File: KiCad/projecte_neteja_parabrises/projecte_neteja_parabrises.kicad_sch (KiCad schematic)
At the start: 0 parts

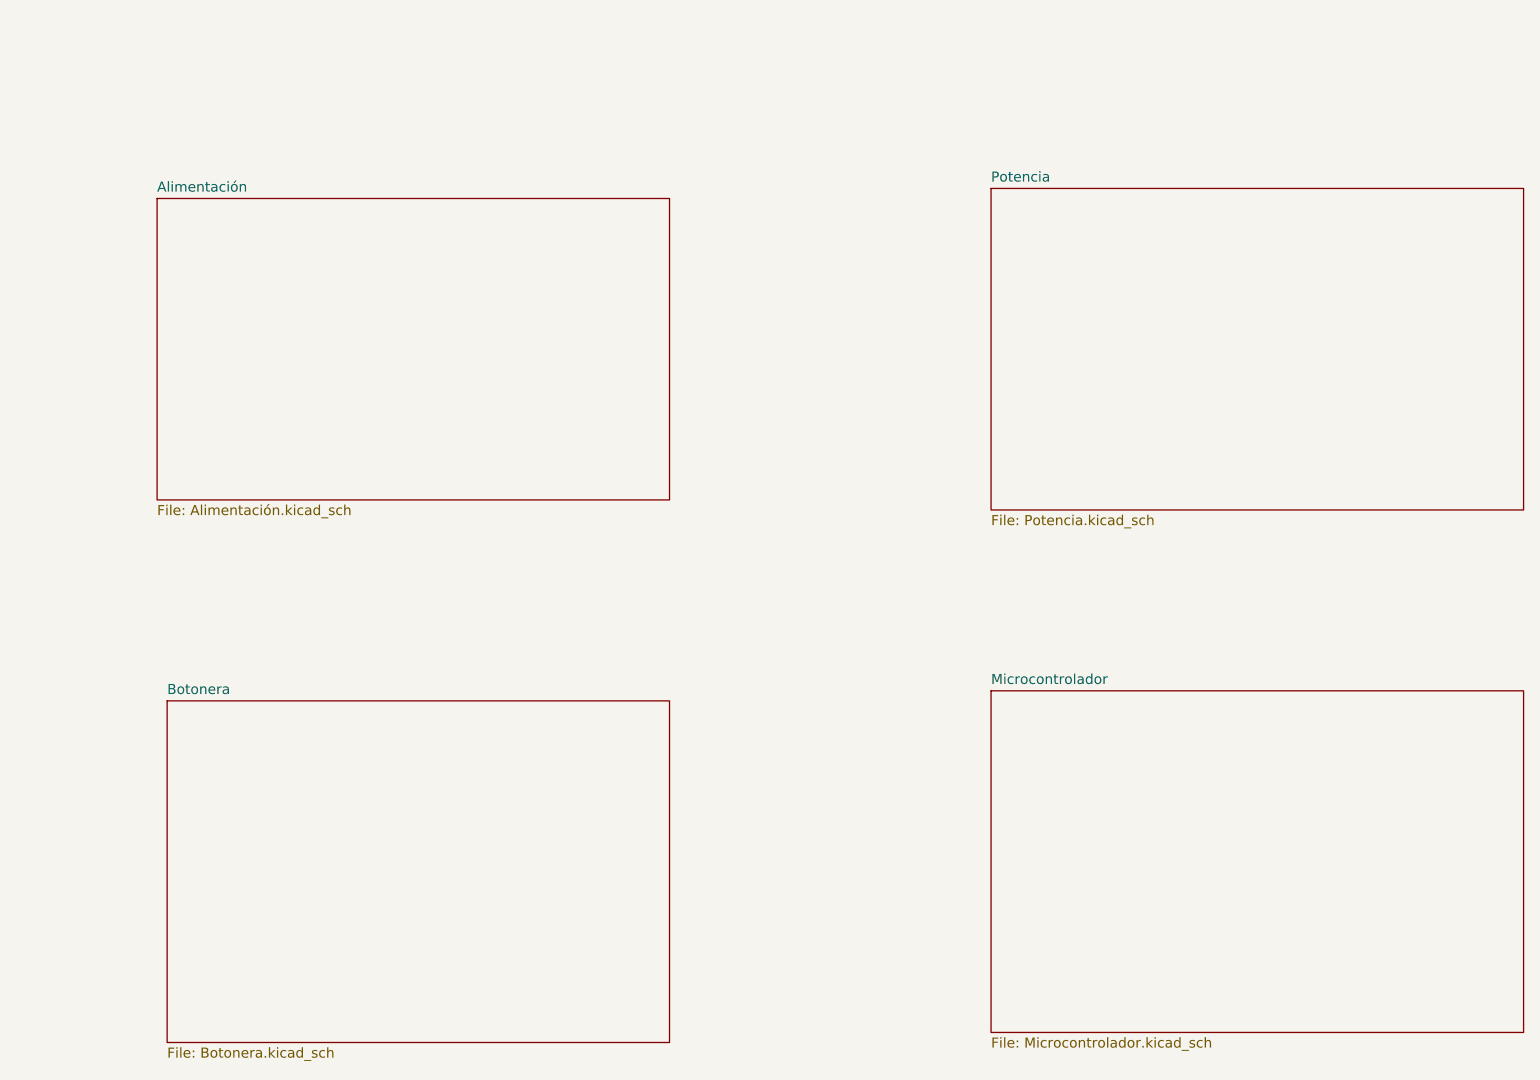
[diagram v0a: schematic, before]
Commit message: ESQUEMATICO V2
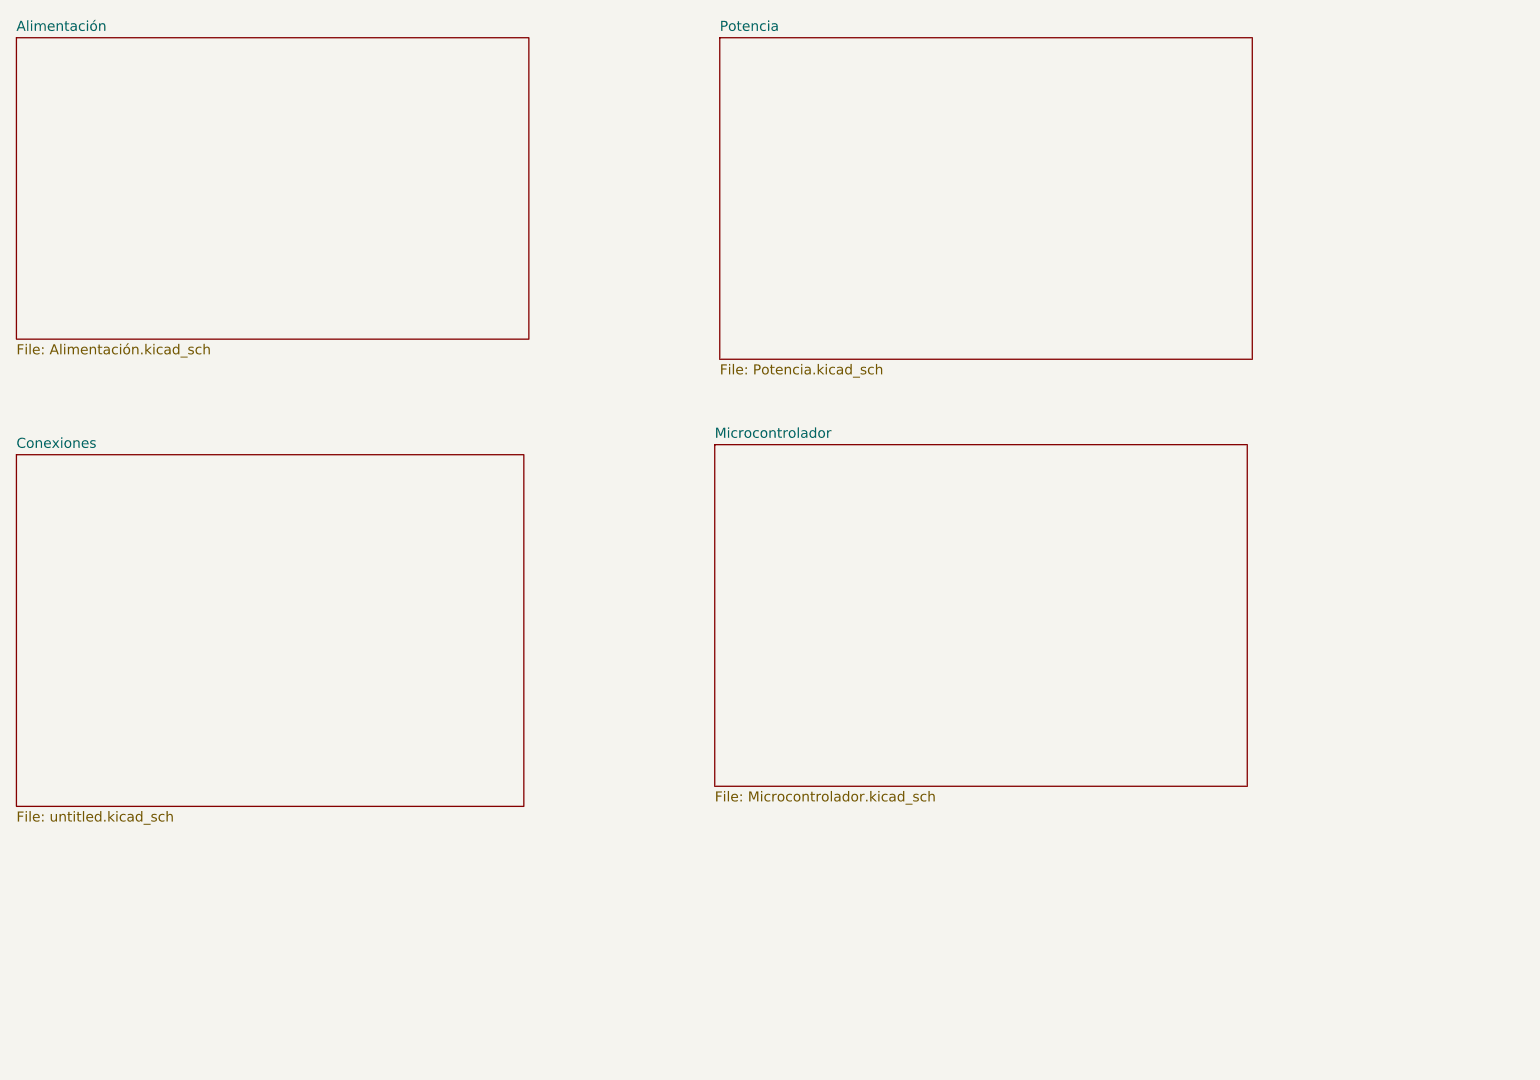
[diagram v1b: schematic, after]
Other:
- removed sheet Botonera
- added sheet Conexiones (untitled.kicad_sch)
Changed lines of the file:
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@@
 	(paper "A4")
 	(sheet
-		(at 40.64 105.41)
-		(size 63.5 43.18)
+		(at 21.59 74.295)
+		(size 64.135 44.45)
 		(exclude_from_sim no)
 		(in_bom yes)
@@
 			(color 0 0 0 0.0000)
 		)
-		(property "Sheetname" "Botonera"
-			(at 40.64 104.6984 0)
+		(property "Sheetname" "Conexiones"
+			(at 21.59 73.5834 0)
 			(effects
 				(font
@@
 			)
 		)
-		(property "Sheetfile" "Botonera.kicad_sch"
-			(at 40.64 149.1746 0)
+		(property "Sheetfile" "untitled.kicad_sch"
+			(at 21.59 119.3296 0)
 			(effects
 				(font
@@
 			)
 		)
+		(property "Field2" ""
+			(at 21.59 74.295 0)
+			(effects
+				(font
+					(size 1.27 1.27)
+				)
+			)
+		)
+		(property "Field3" ""
+			(at 21.59 74.295 0)
+			(effects
+				(font
+					(size 1.27 1.27)
+				)
+			)
+		)
+		(property "Field4" ""
+			(at 21.59 74.295 0)
+			(effects
+				(font
+					(size 1.27 1.27)
+				)
+			)
+		)
+		(property "Field5" ""
+			(at 21.59 74.295 0)
+			(effects
+				(font
+					(size 1.27 1.27)
+				)
+			)
+		)
+		(property "Field6" ""
+			(at 21.59 74.295 0)
+			(effects
+				(font
+					(size 1.27 1.27)
+				)
+			)
+		)
 		(instances
 			(project "projecte_neteja_parabrises"
 				(path "/83fe8808-b70b-463e-9fcd-89556c9690a9"
-					(page "4")
+					(page "6")
 				)
 			)
@@
 	)
 	(sheet
-		(at 144.78 40.64)
+		(at 110.49 21.59)
 		(size 67.31 40.64)
 		(exclude_from_sim no)
@@
 		)
 		(property "Sheetname" "Potencia"
-			(at 144.78 39.9284 0)
+			(at 110.49 20.8784 0)
 			(effects
 				(font
@@
 		)
 		(property "Sheetfile" "Potencia.kicad_sch"
-			(at 144.78 81.8646 0)
+			(at 110.49 62.8146 0)
 			(effects
 				(font
@@
 	)
 	(sheet
-		(at 144.78 104.14)
+		(at 109.855 73.025)
 		(size 67.31 43.18)
 		(exclude_from_sim no)
@@
 		)
 		(property "Sheetname" "Microcontrolador"
-			(at 144.78 103.4284 0)
+			(at 109.855 72.3134 0)
 			(effects
 				(font
@@
 		)
 		(property "Sheetfile" "Microcontrolador.kicad_sch"
-			(at 144.78 147.9046 0)
+			(at 109.855 116.7896 0)
 			(effects
 				(font
@@
 	)
 	(sheet
-		(at 39.37 41.91)
+		(at 21.59 21.59)
 		(size 64.77 38.1)
 		(exclude_from_sim no)
@@
 		)
 		(property "Sheetname" "Alimentación"
-			(at 39.37 41.1984 0)
+			(at 21.59 20.8784 0)
 			(effects
 				(font
@@
 		)
 		(property "Sheetfile" "Alimentación.kicad_sch"
-			(at 39.37 80.5946 0)
+			(at 21.59 60.2746 0)
 			(effects
 				(font
